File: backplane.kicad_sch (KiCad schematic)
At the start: 20 parts, among them J101 USB_C_Receptacle_USB2.0, SW101 RESET, U101 USB2514BI, Y101 24MHZ

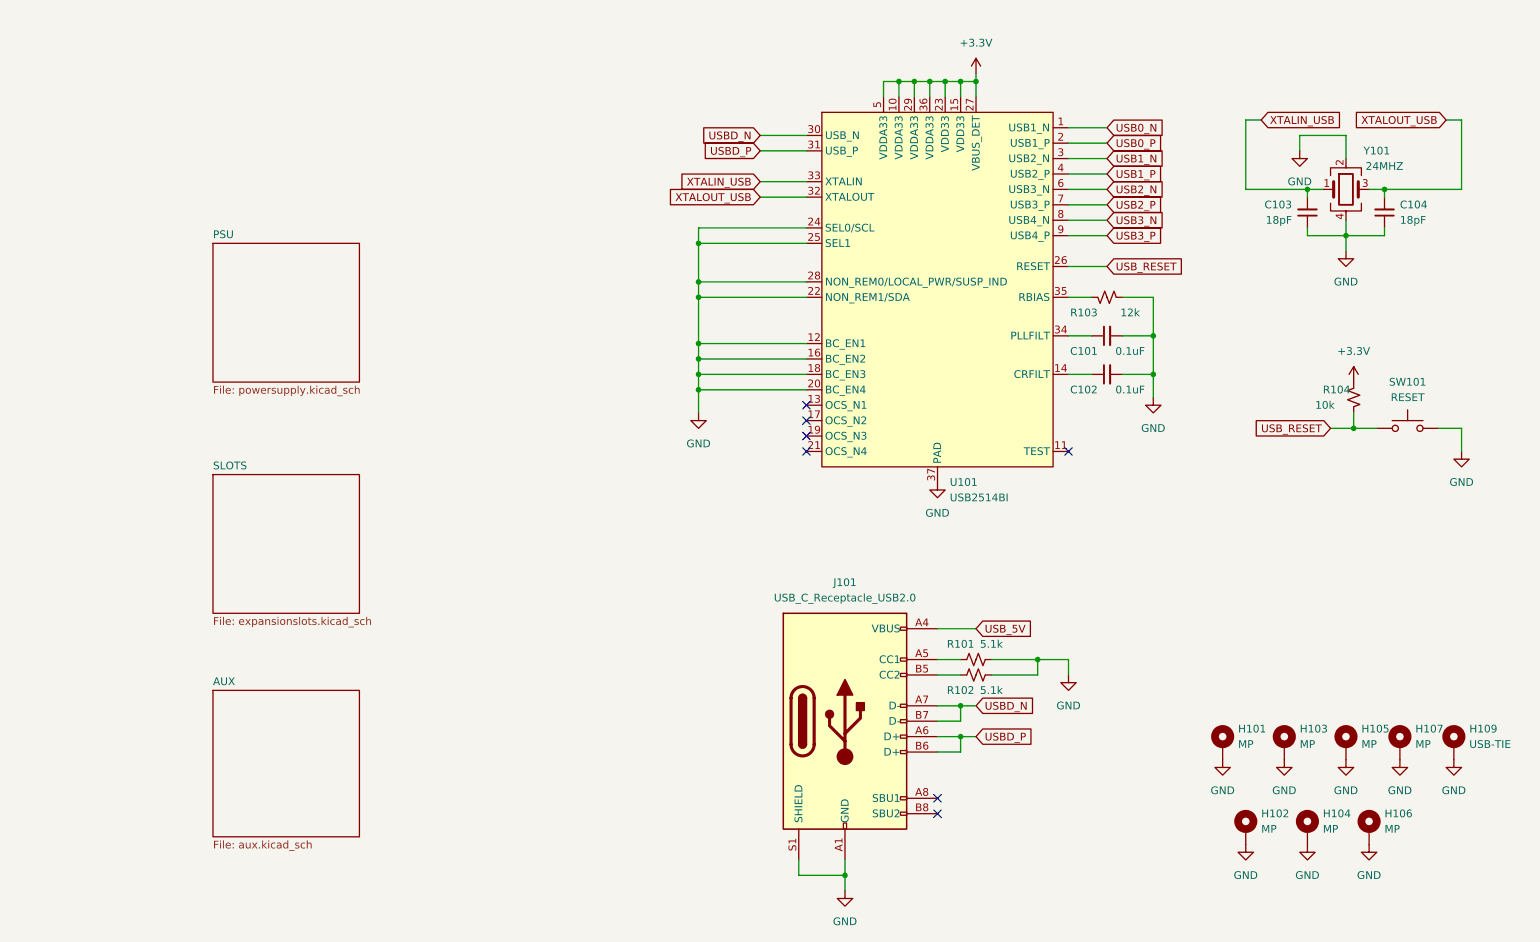
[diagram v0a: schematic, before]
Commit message: update board
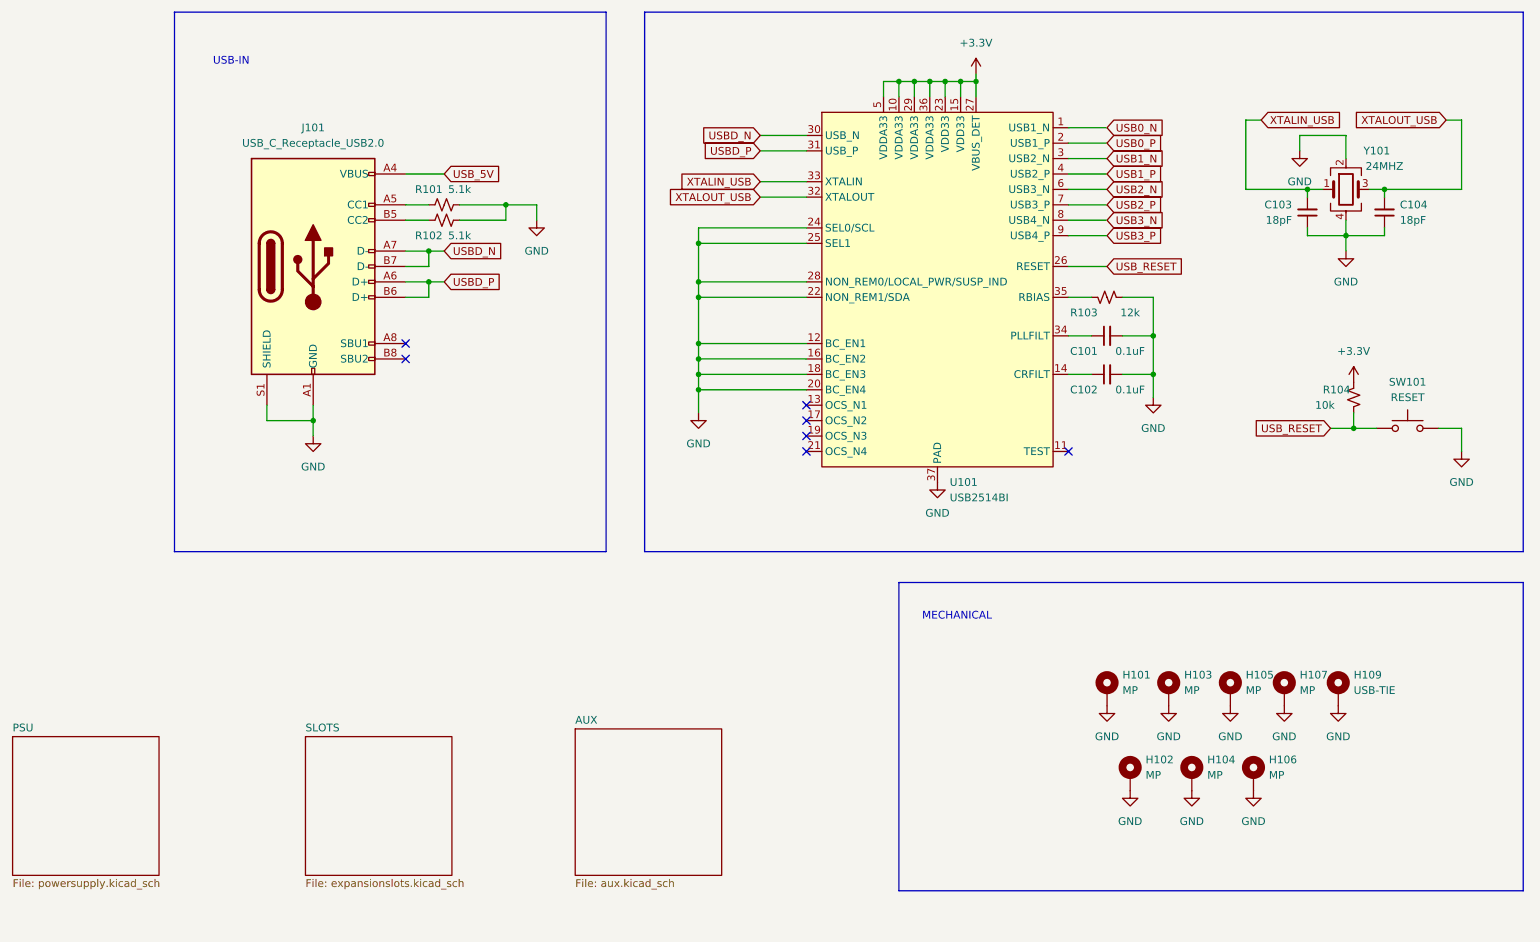
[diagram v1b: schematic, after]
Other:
- note added: "MECHANICAL"
- note added: "USB-IN"
- moved on the sheet: H101, H102, H103, H104, H105, H106, H107, H109, J101, R101, R102
